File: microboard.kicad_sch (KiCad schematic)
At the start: 85 parts, among them J1 Conn_01x01, J10 Conn_01x01, J11 Conn_01x01, J12 Conn_01x10, J13 Conn_01x01, J17 Conn_01x01, J18 Conn_01x01, J2 Conn_01x10, J21 Conn_01x01_Socket, J22 Conn_01x01_Socket, J24 Conn_01x01, J25 Conn_01x01, J3 Conn_02x12, J39 Conn_01x10, J4 USB_C_Receptacle_USB2.0, J40 Conn_01x10, J41 Conn_01x10, J43 Conn_01x05, J44 Conn_01x09, J45 Conn_01x08, J5 Conn_01x04, J6 Conn_01x04, J7 Conn_01x05, J8 Conn_01x10, J9 Conn_01x01, SW1 SW_Push, SW2 SW_Push, SW7 RotaryEncoder_Switch, U1 USBLC6-2SC6, U2 ATSAMD21G18A-AUT, U3 LF33_TO220, U4 TXS0108EPW, U7 LF50_TO220, Y1 32768Hz

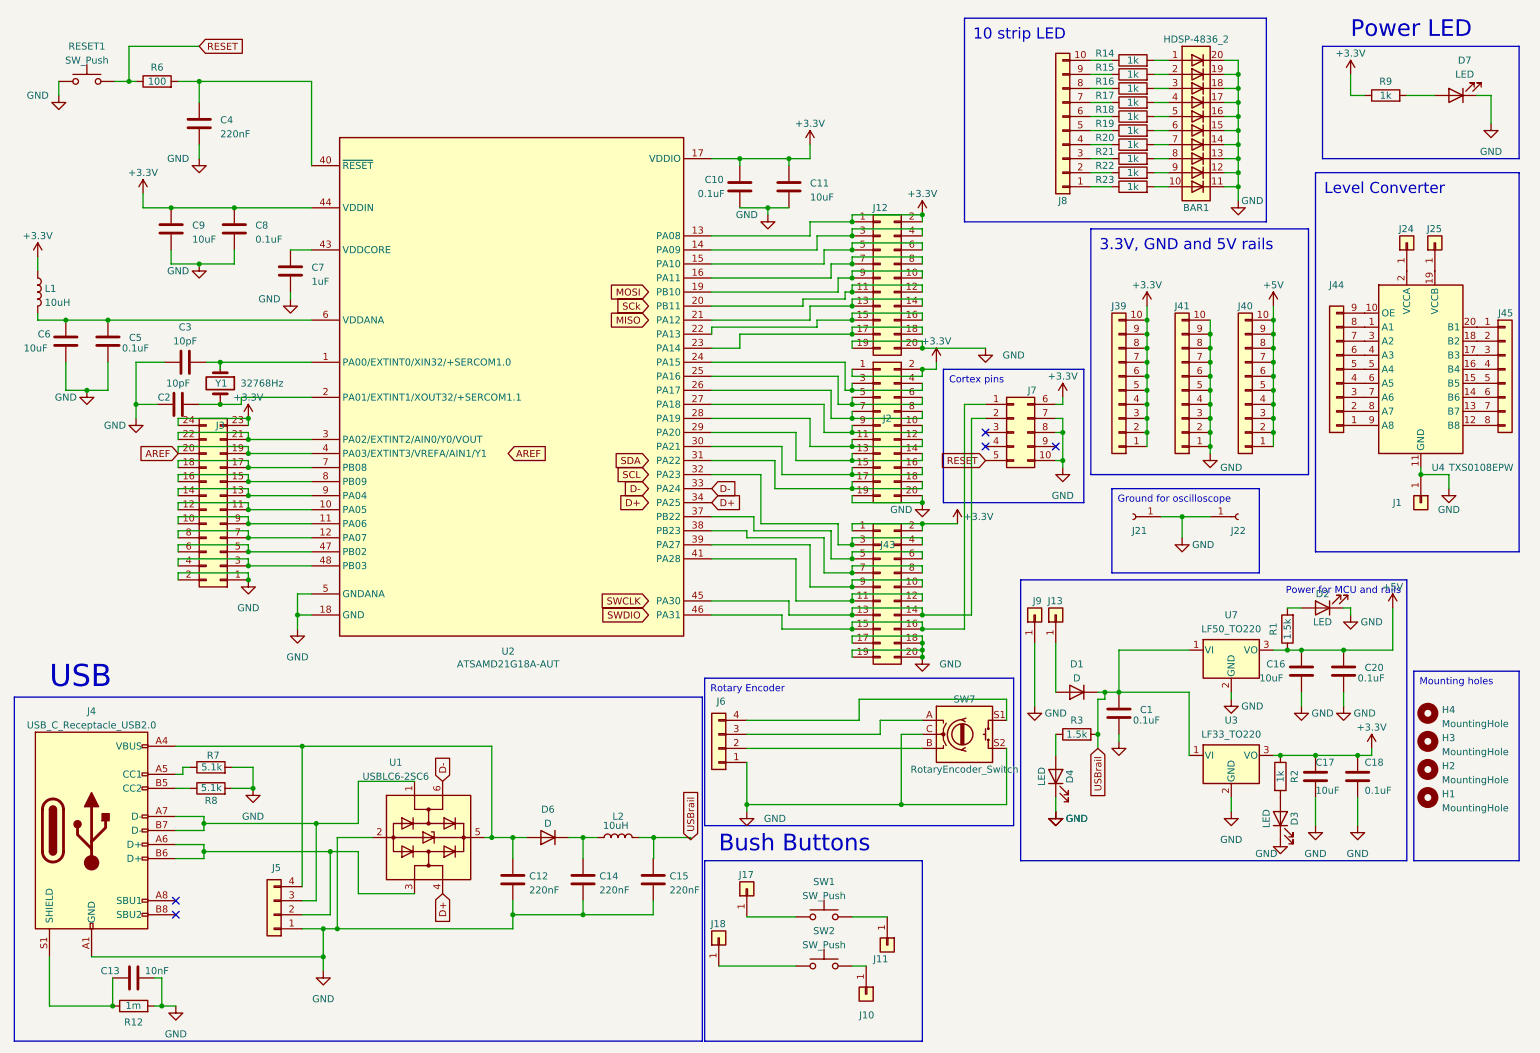
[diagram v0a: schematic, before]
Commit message: paths
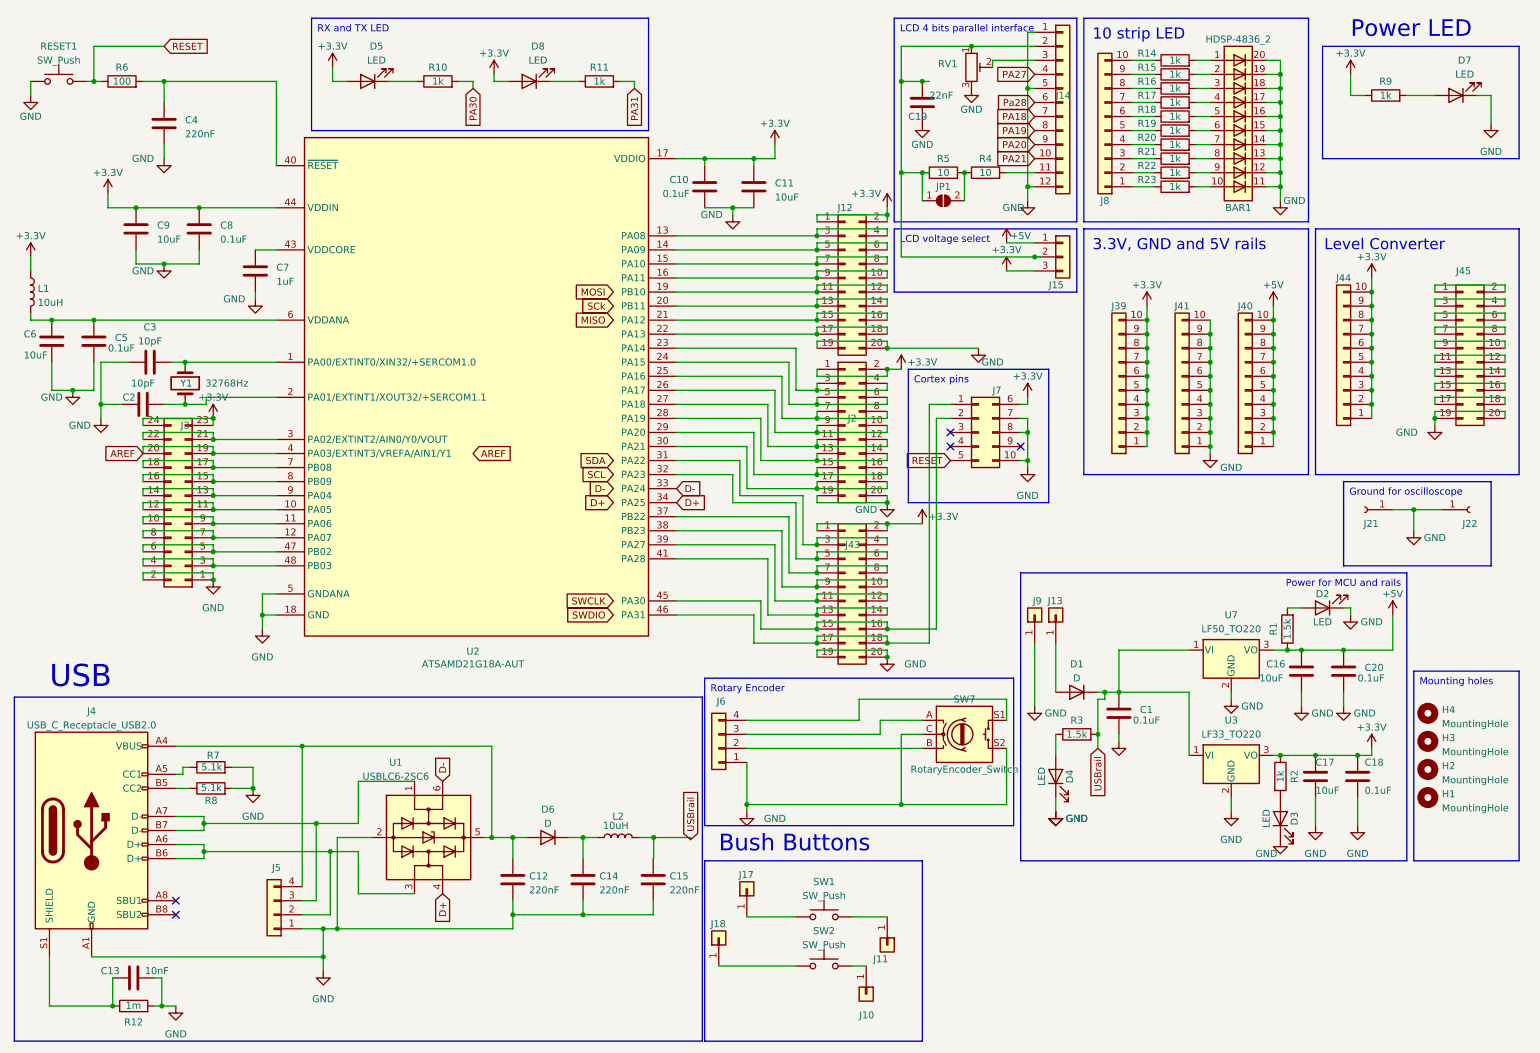
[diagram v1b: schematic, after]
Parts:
- removed J1, J24, J25: Conn_01x01, Connector_PinHeader_2.54mm:PinHeader_1x01_P2.54mm_Vertical, symbol Connector_Generic:Conn_01x01
- removed U4: TXS0108EPW, Package_SO:TSSOP-20_4.4x6.5mm_P0.65mm, symbol Logic_LevelTranslator:TXS0108EPW
- added C19: 22nF, Capacitor_SMD:C_0805_2012Metric_Pad1.18x1.45mm_HandSolder, symbol Device:C
- added D5, D8: LED, LED_SMD:LED_0805_2012Metric_Pad1.15x1.40mm_HandSolder, symbol Device:LED
- added J14: Conn_01x12, Connector_PinHeader_2.54mm:PinHeader_1x12_P2.54mm_Vertical, symbol Connector_Generic:Conn_01x12
- added J15: Conn_01x03, Connector_PinHeader_2.54mm:PinHeader_1x03_P2.54mm_Vertical, symbol Connector_Generic:Conn_01x03
- added JP1: SolderJumper_2_Open, Jumper:SolderJumper-2_P1.3mm_Open_RoundedPad1.0x1.5mm, symbol Jumper:SolderJumper_2_Open
- added R10, R11: 1k, Resistor_SMD:R_0805_2012Metric_Pad1.20x1.40mm_HandSolder, symbol Device:R
- added R4, R5: 10, Resistor_SMD:R_0805_2012Metric_Pad1.20x1.40mm_HandSolder, symbol Device:R
- added RV1: R_Potentiometer_Trim, Potentiometer_THT:Potentiometer_Runtron_RM-065_Vertical, symbol Device:R_Potentiometer_Trim
- J44: footprint Connector_PinHeader_2.54mm:PinHeader_1x09_P2.54mm_Vertical -> Connector_PinHeader_2.54mm:PinHeader_1x10_P2.54mm_Vertical; symbol Connector_Generic:Conn_01x09 -> Connector_Generic:Conn_01x10
- J45: footprint Connector_PinHeader_2.54mm:PinHeader_1x08_P2.54mm_Vertical -> Connector_PinHeader_2.54mm:PinHeader_2x10_P2.54mm_Vertical; symbol Connector_Generic:Conn_01x08 -> Connector_Generic:Conn_02x10_Odd_Even
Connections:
- net +3.3V: now also J44.1 (Pin_1), J44.10 (Pin_10), J44.2 (Pin_2), J44.3 (Pin_3), J44.4 (Pin_4), J44.5 (Pin_5), J44.6 (Pin_6), J44.7 (Pin_7), J44.8 (Pin_8), J44.9 (Pin_9), D5.2 (A), D8.2 (A), J15.3 (Pin_3); no longer U2.13 (PA08)
- net +5V: now also J15.1 (Pin_1)
- net GND: now also J45.19 (Pin_19), J45.20 (Pin_20), C19.2, J14.1 (Pin_1), J14.12 (Pin_12), J14.5 (Pin_5), RV1.3; no longer J43.17 (Pin_17), J43.18 (Pin_18)
- net at J43.10 (Pin_10), J43.9 (Pin_9): now also U2.38 (PB23); no longer U2.39 (PA27)
- net at J43.11 (Pin_11), J43.12 (Pin_12): now also U2.39 (PA27); no longer U2.41 (PA28)
- net at J43.13 (Pin_13), J43.14 (Pin_14): now also U2.41 (PA28); no longer J7.2 (Pin_2), U2.45 (PA30)
- net at J43.15 (Pin_15), J43.16 (Pin_16): now also J7.2 (Pin_2), U2.45 (PA30); no longer J7.1 (Pin_1), U2.46 (PA31)
- net at J43.3 (Pin_3), J43.4 (Pin_4): now also U2.31 (PA22); no longer U2.32 (PA23)
- net at J43.5 (Pin_5), J43.6 (Pin_6): now also U2.32 (PA23); no longer U2.37 (PB22)
- net at J43.7 (Pin_7), J43.8 (Pin_8): now also U2.37 (PB22); no longer U2.38 (PB23)
- net at J12.10 (Pin_10), J12.9 (Pin_9): now also U2.16 (PA11); no longer U2.19 (PB10)
- net at J12.11 (Pin_11), J12.12 (Pin_12): now also U2.19 (PB10); no longer U2.20 (PB11)
- net at J12.13 (Pin_13), J12.14 (Pin_14): now also U2.20 (PB11); no longer U2.21 (PA12)
- net at J12.15 (Pin_15), J12.16 (Pin_16): now also U2.21 (PA12); no longer U2.22 (PA13)
- net at J12.17 (Pin_17), J12.18 (Pin_18): now also U2.22 (PA13); no longer U2.23 (PA14)
- net at J12.3 (Pin_3), J12.4 (Pin_4): now also U2.13 (PA08); no longer U2.14 (PA09)
- net at J12.5 (Pin_5), J12.6 (Pin_6): now also U2.14 (PA09); no longer U2.15 (PA10)
- net at J12.7 (Pin_7), J12.8 (Pin_8): now also U2.15 (PA10); no longer U2.16 (PA11)
- net at J2.3 (Pin_3), J2.4 (Pin_4): now also U2.23 (PA14); no longer U2.24 (PA15)
- net at J2.5 (Pin_5), J2.6 (Pin_6): now also U2.24 (PA15); no longer U2.25 (PA16)
- net at J2.7 (Pin_7), J2.8 (Pin_8): now also U2.25 (PA16); no longer U2.26 (PA17)
- net at J2.10 (Pin_10), J2.9 (Pin_9): now also U2.26 (PA17); no longer U2.27 (PA18)
- net at J2.11 (Pin_11), J2.12 (Pin_12): now also U2.27 (PA18); no longer U2.28 (PA19)
- net at J2.13 (Pin_13), J2.14 (Pin_14): now also U2.28 (PA19); no longer U2.29 (PA20)
- net at J2.15 (Pin_15), J2.16 (Pin_16): now also U2.29 (PA20); no longer U2.30 (PA21)
- net at J2.17 (Pin_17), J2.18 (Pin_18): now also U2.30 (PA21); no longer U2.31 (PA22)
- net at J45.1 (Pin_1): now also J45.2 (Pin_2)
- net at J45.3 (Pin_3): now also J45.4 (Pin_4)
- net at J45.5 (Pin_5): now also J45.6 (Pin_6)
- net at J45.7 (Pin_7): now also J45.8 (Pin_8)
- new net: J43.17 (Pin_17), J43.18 (Pin_18), J7.1 (Pin_1), U2.46 (PA31)
- new net: C19.1, J14.2 (Pin_2), J15.2 (Pin_2), JP1.1 (A), R5.1, RV1.1
- new net: J14.3 (Pin_3), RV1.2
- new net: JP1.2 (B), R4.1, R5.2
- new net: D5.1 (K), R10.1
- new net: J14.11 (Pin_11), R4.2
- new net: J45.10 (Pin_10), J45.9 (Pin_9)
- new net: J45.11 (Pin_11), J45.12 (Pin_12)
- new net: J45.13 (Pin_13), J45.14 (Pin_14)
- new net: J45.15 (Pin_15), J45.16 (Pin_16)
- new net: J45.17 (Pin_17), J45.18 (Pin_18)
- new net: D8.1 (K), R11.1
- new net PA18: J14.7 (Pin_7)
- new net PA19: J14.8 (Pin_8)
- new net PA20: J14.9 (Pin_9)
- new net PA21: J14.10 (Pin_10)
- new net PA27: J14.4 (Pin_4)
- new net PA30: R10.2
- new net PA31: R11.2
- new net Pa28: J14.6 (Pin_6)
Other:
- moved on the sheet: BAR1, C10, C11, C2, C3, C4, C5, C6, C7, C8, C9, J12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
